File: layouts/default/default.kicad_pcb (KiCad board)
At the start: 4 copper layers, 54 x 57.2 mm, 52 parts

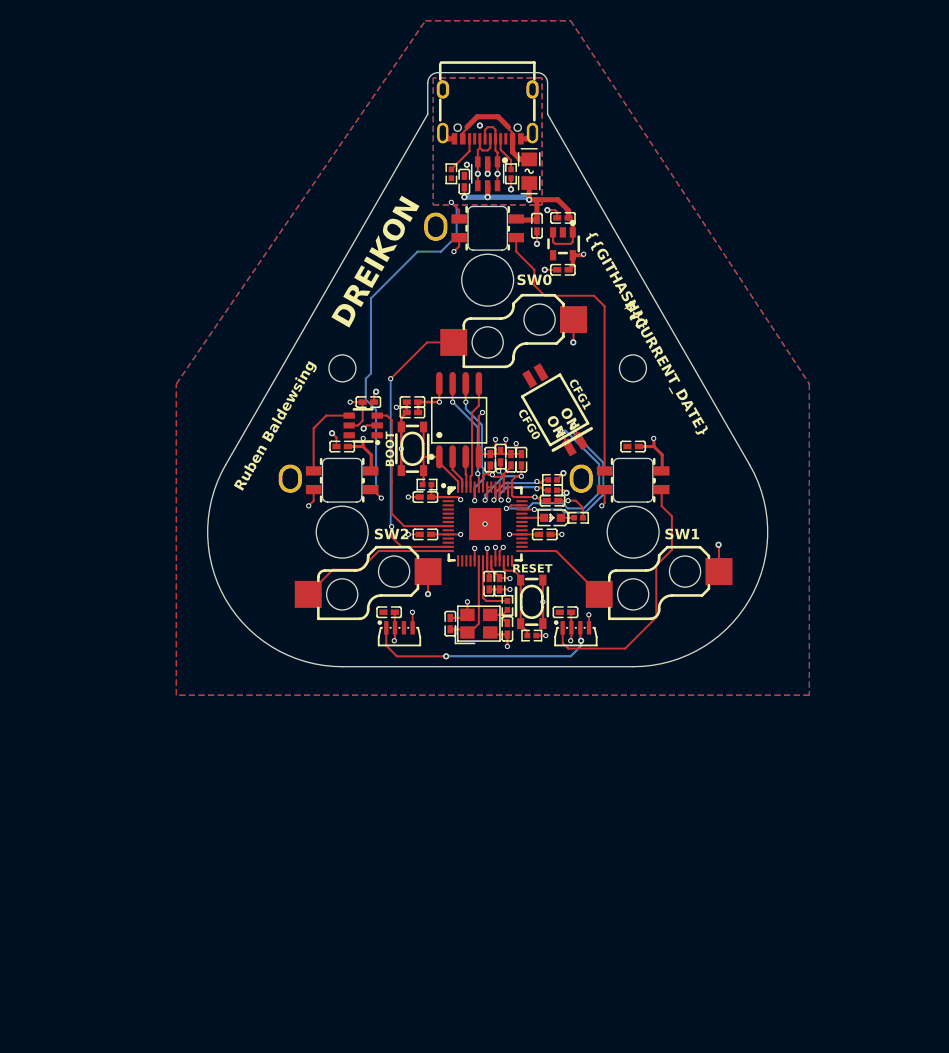
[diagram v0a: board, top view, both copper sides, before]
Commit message: feat(PCB): Finish routing
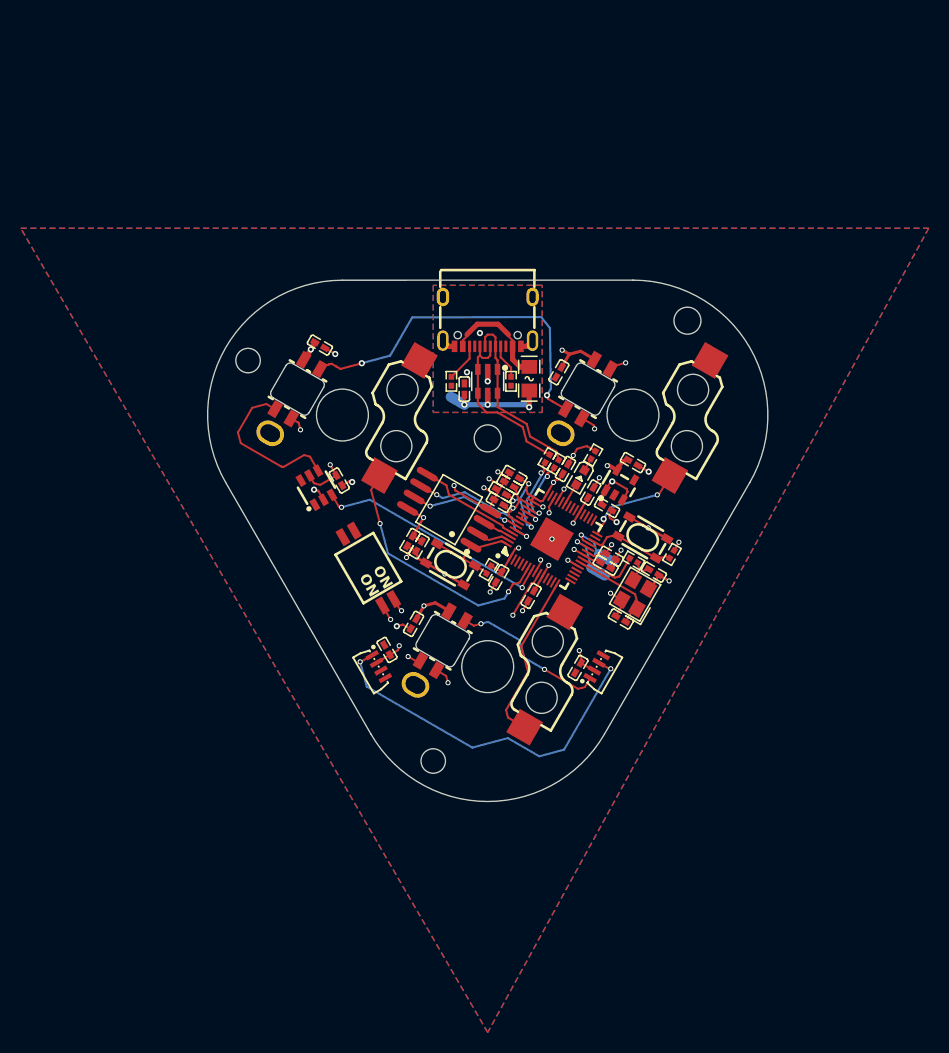
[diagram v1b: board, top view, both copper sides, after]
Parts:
- moved LOGO1 29.9 mm to (-0.25, 46.7)
- moved C18 28.2 mm to (11.5, 21.9), turned to -30 degrees
- moved LED1 24.0 mm to (-18.3, 10.5), turned to -30 degrees
- moved U7 23.9 mm to (12.8, 19.7), turned to -120 degrees
- moved C1 23.9 mm to (-16.2, 6.26), turned to -30 degrees
- moved SW3 23.6 mm to (-11.5, 27.7)
- moved R8 20.0 mm to (-3.50, 9.75)
- moved USB1 20.0 mm to (0.00, 4.00)
- moved D1 20.0 mm to (0.00, 9.75)
- moved R7 20.0 mm to (2.25, 9.75)
- moved C20 20.0 mm to (-2.25, 10.5)
- moved F1 20.0 mm to (4.00, 9.50)
- moved C19 19.8 mm to (14.0, 17.6), turned to -30 degrees
- moved LED5 19.4 mm to (10.5, 37.2), turned to -120 degrees
- moved LED6 19.4 mm to (-10.5, 37.2), turned to 120 degrees
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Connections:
- LED1 pad 4: led_data_out-line -> switches[0]-led_data_in-line
- LED2 pad 2: led_data_out-DIN -> switches[2]-led_data_in-line
- LED3 pad 2: led_data_out-line -> led_data_out-DIN
- LED5 pad 1: data_out-DIN -> led_data_out-DIN
- LED5 pad 3: DOUT -> data_in-DIN
- LED6 pad 1: led_data_out-DIN -> data_in-DIN
- LED6 pad 3: data_out-DIN -> DOUT
- SW3 pad 1: gpio[28]-line -> gpio[7]-line
- SW3 pad 2: gpio[27]-line -> gpio[6]-line
- U2 pad 1: SCLK -> switches[1]-output-contact[0]
- U5 pad 13: switches[0]-output-contact[0] -> GPIO10
- U5 pad 28: GPIO17 -> switches[1]-output-contact[0]
- U5 pad 6: GPIO4 -> switches[0]-output-contact[0]
- U5 pad 7: GPIO5 -> gpio[5]-line
- U5 pad 9: GPIO7 -> gpio[7]-line
- U8 pad 3: gpio[6]-line -> gpio[5]-line
- U8 pad 4: switches[2]-led_data_in-line -> switches[0]-led_data_in-line
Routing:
- net switches[2]-led_data_in-line: track 8.04 -> 63.2 mm, vias 0 -> 2
- net led_data_out-line: track 37.5 -> 0.00 mm, vias 2 -> 0
- net data_in-DIN: track 0.00 -> 35.4 mm, vias 0 -> 2
- net input-USB_D_N: track 50.8 -> 17.2 mm, vias 2 -> 0
- net input-USB_D_P: track 47.2 -> 16.7 mm, vias 2 -> 0
- net gpio[5]-line: track 0.00 -> 23.3 mm, vias 0 -> 2
- net data_out-DIN: track 23.1 -> 0.00 mm, vias 2 -> 0
- net gpio[7]-line: track 0.00 -> 19.8 mm, vias 0 -> 2
- net gpio[28]-line: track 21.3 -> 1.62 mm, vias 2 -> 1
- net gpio[27]-line: track 18.2 -> 1.20 mm, vias 2 -> 1
- net switches[0]-led_data_in-line: track 0.00 -> 15.4 mm
- net GND: track 68.3 -> 57.5 mm, vias 34 -> 28
- net led_data_out-DIN: track 25.3 -> 15.3 mm, vias 0 -> 2
- net switches[1]-output-contact[0]: track 0.00 -> 9.89 mm, vias 0 -> 2
- net SCLK: track 9.20 -> 0.00 mm
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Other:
- board size 54 x 57.2 mm -> 54 x 50.2 mm
- board text added: "5V"
- board text added: "CLK"
- board text added: "DIO"
- board text added: "GND"
- board text added: "SWITCH 0"
- board text added: "SWITCH 1"
- board text added: "SWITCH 2"
- board text removed: "SW0"
- board text removed: "SW1"
- board text removed: "SW2"
